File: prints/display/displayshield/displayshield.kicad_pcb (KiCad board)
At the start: 2 copper layers, 123 x 61 mm, 13 parts, among them J1 Display, J2 RaspberryPiDisplay, J3 RaspberryPiADC, J4 CurrentSensor, SW1 SW_Push

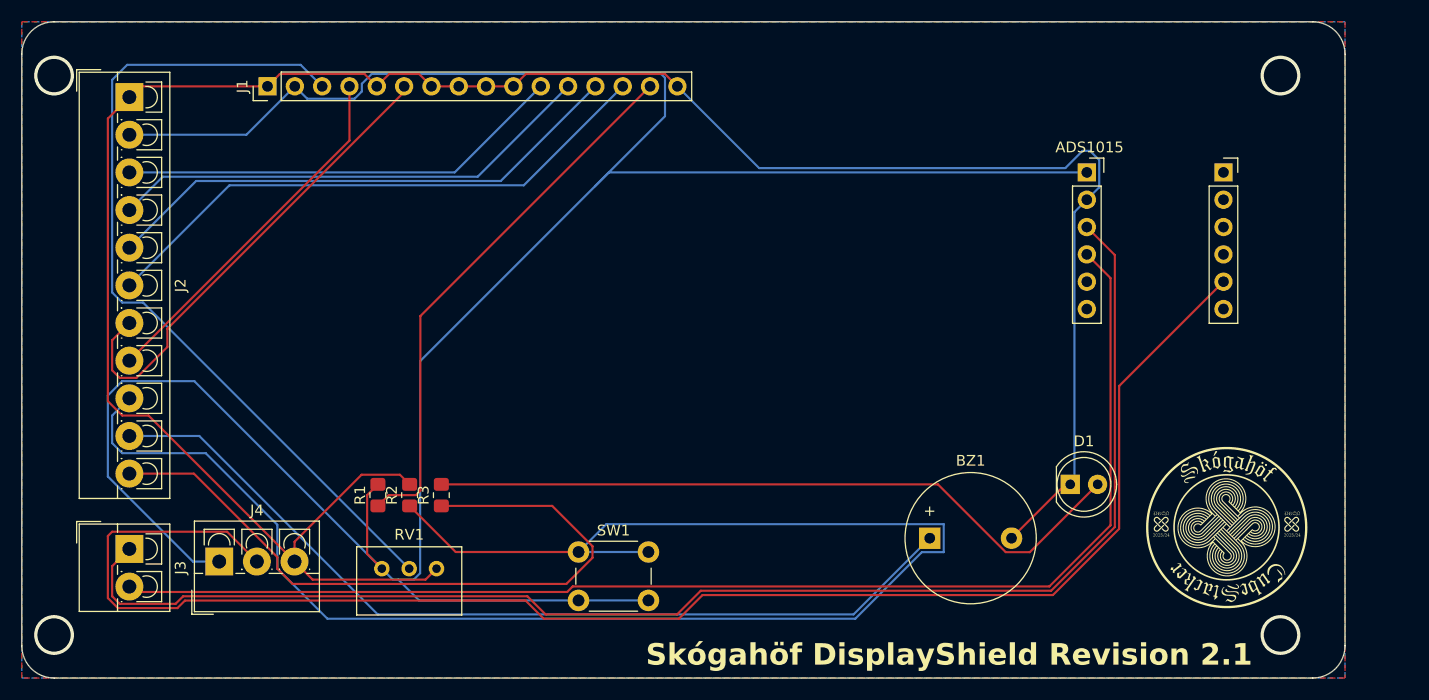
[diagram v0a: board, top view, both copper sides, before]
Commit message: updated StackMeasurements
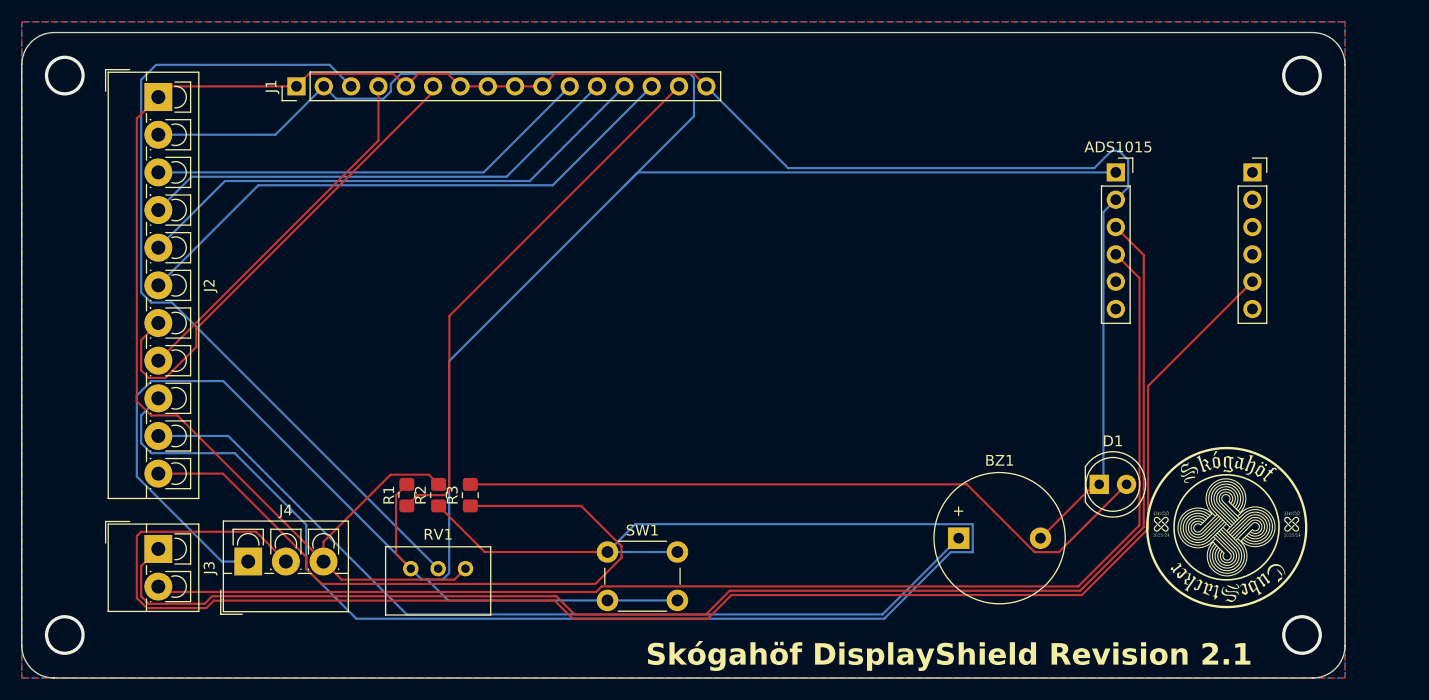
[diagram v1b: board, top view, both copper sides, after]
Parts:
- moved ADS1015 2.69 mm to (211.4, 73.2)
- moved J2 2.69 mm to (115.7, 62.0)
- moved J3 2.69 mm to (115.7, 104.0)
- moved J4 2.69 mm to (124.0, 105.2)
- moved BZ1 2.69 mm to (190.1, 103.0)
- moved D1 2.69 mm to (203.2, 98.0)
- moved J1 2.69 mm to (128.5, 61.0)
- moved R1 2.69 mm to (138.8, 99.0)
- moved R2 2.69 mm to (141.7, 99.0)
- moved R3 2.69 mm to (144.7, 99.0)
- moved RV1 2.69 mm to (144.2, 105.8)
- moved SW1 2.69 mm to (157.4, 104.3)
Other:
- board size 123 x 61 mm -> 123 x 60 mm
